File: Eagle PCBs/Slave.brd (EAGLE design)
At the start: 56.8 x 35.6 mm, 9 parts

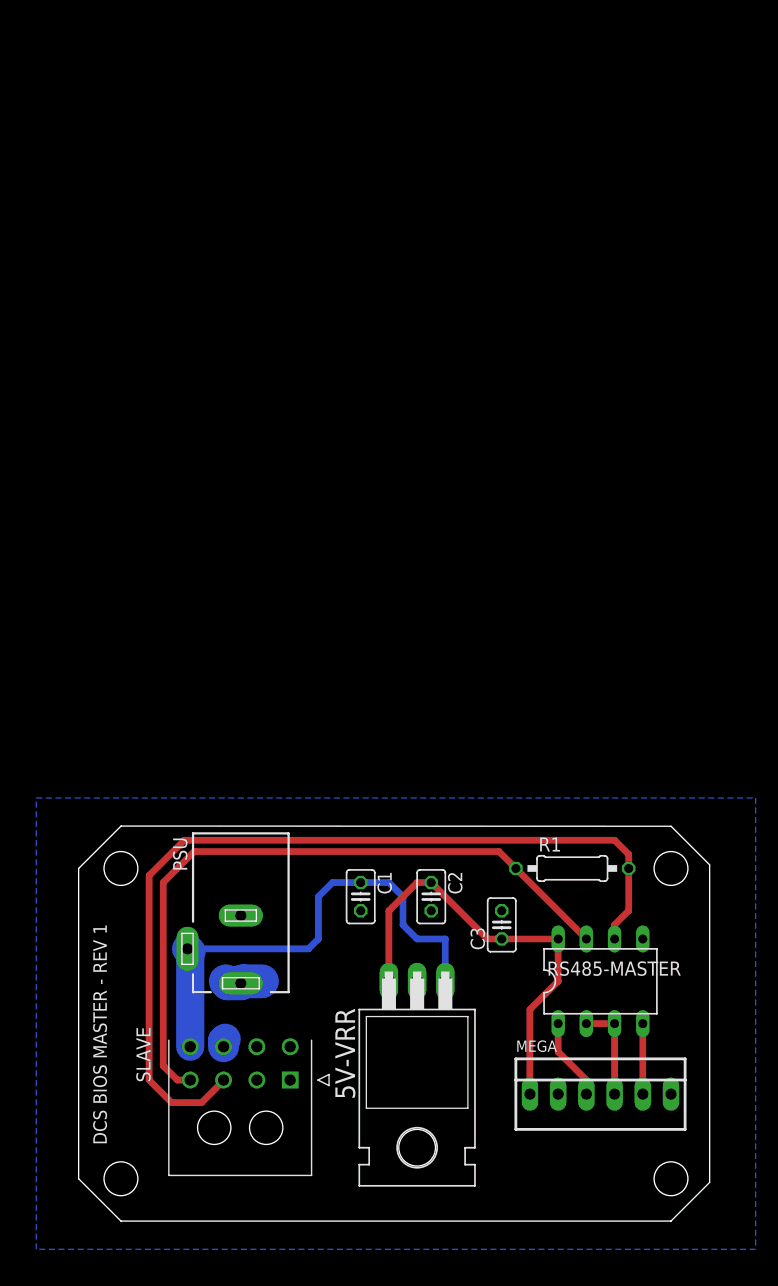
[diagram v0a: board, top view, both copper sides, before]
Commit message: Master PCB WIP
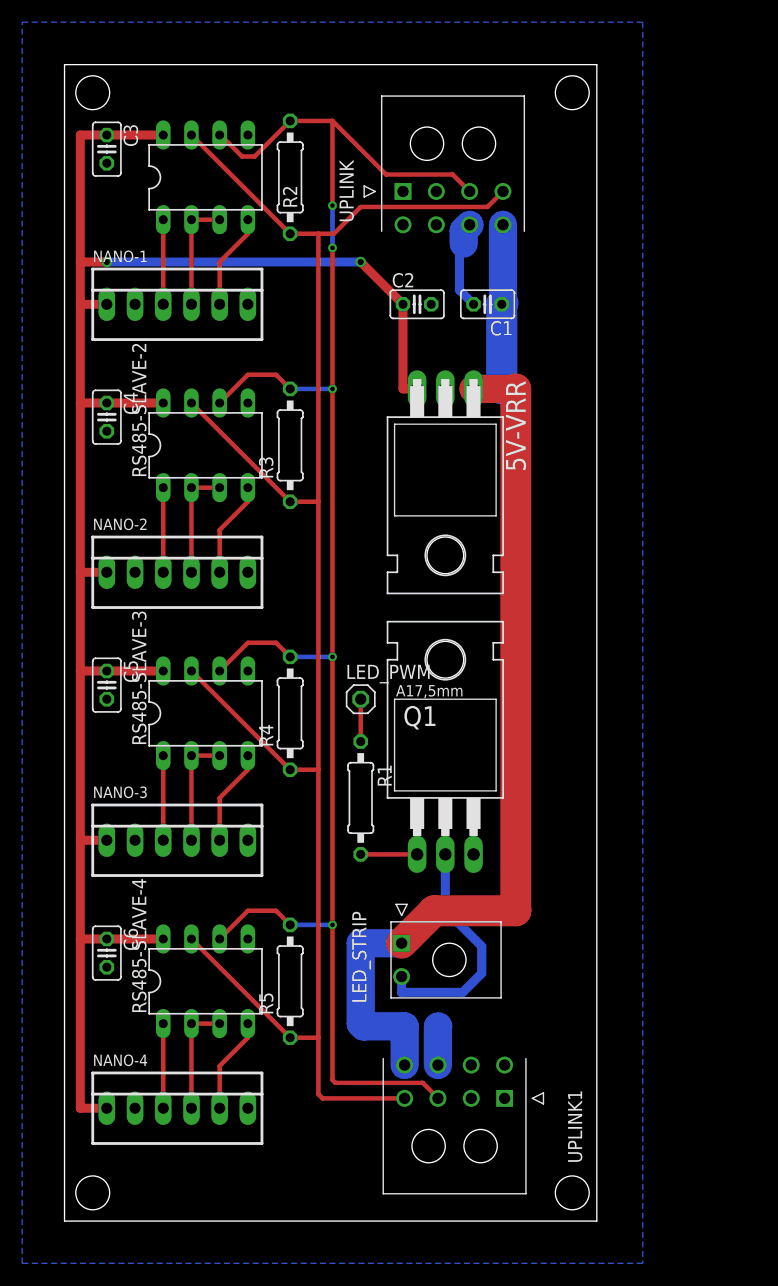
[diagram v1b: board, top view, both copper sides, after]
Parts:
- removed MEGA: (no value), con-molex:22-23-2061
- removed PSU: 12VDC C+, con-jack:DCJ0202
- removed RS485-MASTER: MAX487CPA, A10 Library:DIL08
- removed SLAVE: 212528-0801, SamacSys_Parts:212528-08YY
- added C4, C5, C6: 0.1uF, rcl:C025-025X050
- added LED_PWM: Header, pinhead:1X01
- added LED_STRIP: 215760-3002, SamacSys_Parts:215760-YY02
- added NANO-1, NANO-2, NANO-3, NANO-4: 6P, con-molex:22-23-2061
- added Q1: TIP120, transistor-power:TO220AH
- added R2, R3, R4, R5: 120Ω OPT, rcl:0207/10
- added RS485-SLAVE-1, RS485-SLAVE-2, RS485-SLAVE-3, RS485-SLAVE-4: MAX487CPA, A10 Library:DIL08
- added UPLINK, UPLINK1: 212528-0801, SamacSys_Parts:212528-08YY
- R1: value 120Ω -> 2.2k
- moved C3 78.4 mm to (3.81, 96.5), turned to 270 degrees
- moved C1 54.6 mm to (38.1, 82.5), turned to 180 degrees
- moved 5V-VRR 53.4 mm to (34.3, 64.8)
- moved C2 53.4 mm to (31.8, 82.5), turned to 0 degrees
- moved R1 20.1 mm to (26.7, 38.1), turned to 270 degrees
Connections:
- removed net MEGA_P18: MEGA.5, RS485-MASTER.4
- removed net MEGA_P19: MEGA.3, RS485-MASTER.1
- removed net MEGA_P2: MEGA.4, RS485-MASTER.2, RS485-MASTER.3
- new net DIMMER_PWM_PIN: LED_PWM.1, R1.1
- new net LED_GND: LED_STRIP.2, Q1.C
- new net N$1: Q1.B, R1.2
- new net NANO_1_P2: NANO-1.4, RS485-SLAVE-1.2, RS485-SLAVE-1.3
- new net NANO_1_RX: NANO-1.3, RS485-SLAVE-1.1
- new net NANO_1_TX: NANO-1.5, RS485-SLAVE-1.4
- new net NANO_2_P2: NANO-2.4, RS485-SLAVE-2.2, RS485-SLAVE-2.3
- new net NANO_2_RX: NANO-2.3, RS485-SLAVE-2.1
- new net NANO_2_TX: NANO-2.5, RS485-SLAVE-2.4
- new net NANO_3_P2: NANO-3.4, RS485-SLAVE-3.2, RS485-SLAVE-3.3
- new net NANO_3_RX: NANO-3.3, RS485-SLAVE-3.1
- new net NANO_3_TX: NANO-3.5, RS485-SLAVE-3.4
- new net NANO_4_P2: NANO-4.4, RS485-SLAVE-4.2, RS485-SLAVE-4.3
- new net NANO_4_RX: NANO-4.3, RS485-SLAVE-4.1
- new net NANO_4_TX: NANO-4.5, RS485-SLAVE-4.4
- net GND: now also C4.2, C5.2, C6.2, NANO-1.2, NANO-2.2, NANO-3.2, NANO-4.2, Q1.E, RS485-SLAVE-1.5, RS485-SLAVE-2.5, RS485-SLAVE-3.5, RS485-SLAVE-4.5, UPLINK.7, UPLINK1.7; no longer MEGA.2, PSU.1, RS485-MASTER.5, SLAVE.7
- net RS485_A: now also R2.2, R3.2, R4.2, R5.2, RS485-SLAVE-1.6, RS485-SLAVE-2.6, RS485-SLAVE-3.6, RS485-SLAVE-4.6, UPLINK.3, UPLINK1.3; no longer R1.2, RS485-MASTER.6, SLAVE.3
- net RS485_B: now also R2.1, R3.1, R4.1, R5.1, RS485-SLAVE-1.7, RS485-SLAVE-2.7, RS485-SLAVE-3.7, RS485-SLAVE-4.7, UPLINK.4, UPLINK1.4; no longer R1.1, RS485-MASTER.7, SLAVE.4
- net VCC: now also C4.1, C5.1, C6.1, NANO-1.1, NANO-2.1, NANO-3.1, NANO-4.1, RS485-SLAVE-1.8, RS485-SLAVE-2.8, RS485-SLAVE-3.8, RS485-SLAVE-4.8; no longer MEGA.1, RS485-MASTER.8
- net VCC12: now also LED_STRIP.1, UPLINK.8, UPLINK1.8; no longer PSU.2, SLAVE.8
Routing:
- net VCC: track 39.8 -> 166.6 mm, vias 0 -> 2
- net RS485_B: track 62.0 -> 164.0 mm
- net RS485_A: track 80.0 -> 159.0 mm, vias 0 -> 5
- net VCC12: track 44.2 -> 98.1 mm
- net LED_GND: track 0.00 -> 21.5 mm
- net NANO_2_P2: track 0.00 -> 10.2 mm
- net NANO_1_P2: track 0.00 -> 10.2 mm
- net NANO_4_P2: track 0.00 -> 10.2 mm
- net NANO_3_P2: track 0.00 -> 10.2 mm
- net MEGA_P2: track 8.89 -> 0.00 mm
- net NANO_2_TX: track 0.00 -> 8.67 mm
- net NANO_1_TX: track 0.00 -> 8.67 mm
- net NANO_4_TX: track 0.00 -> 8.67 mm
- net NANO_3_TX: track 0.00 -> 8.67 mm
- net NANO_2_RX: track 0.00 -> 7.62 mm
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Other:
- board size 56.8 x 35.6 mm -> 47.9 x 104.1 mm
- board text removed: "DCS BIOS MASTER - REV 1"
